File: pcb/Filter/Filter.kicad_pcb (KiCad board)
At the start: 2 copper layers, 100 x 100 mm, 8 parts, among them J1 Conn_01x01, J2 Conn_01x01, J3 Conn_01x02

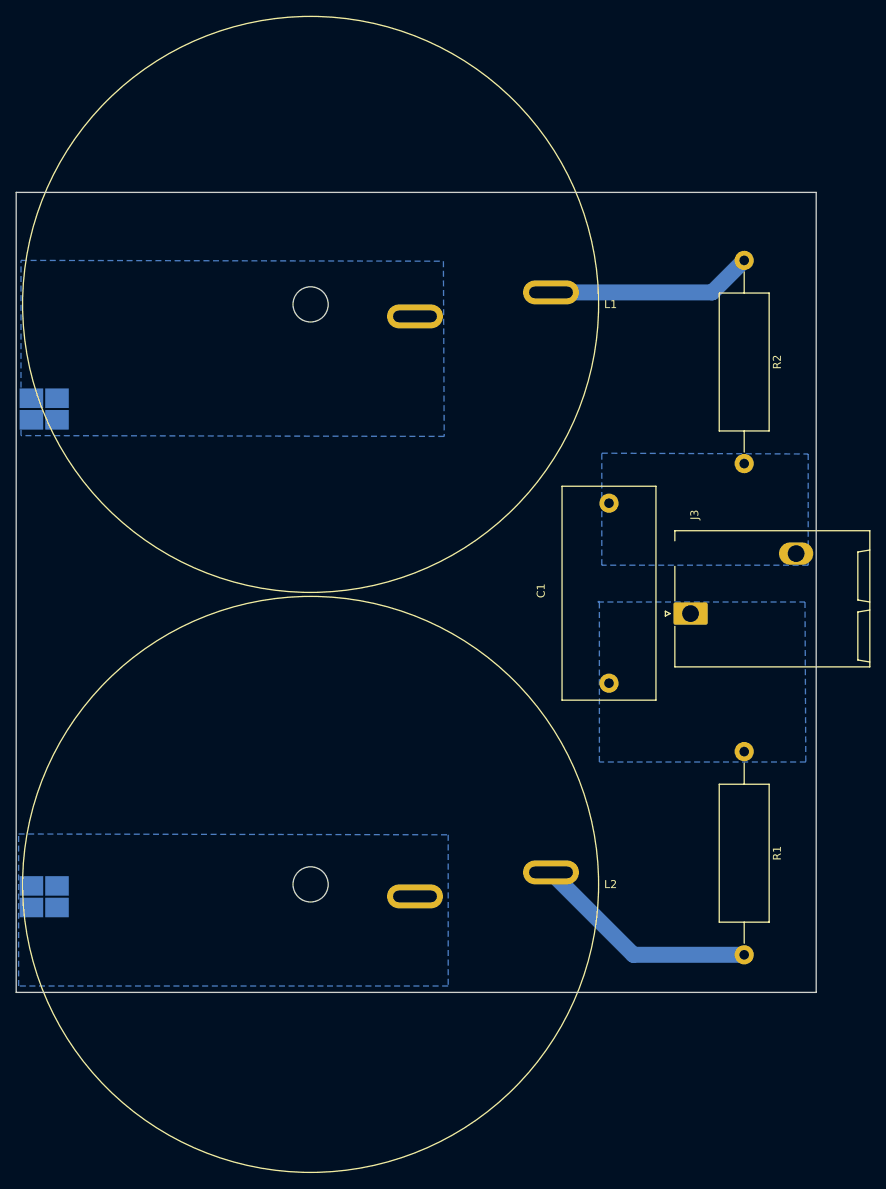
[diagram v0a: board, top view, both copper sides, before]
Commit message: filter + backplane
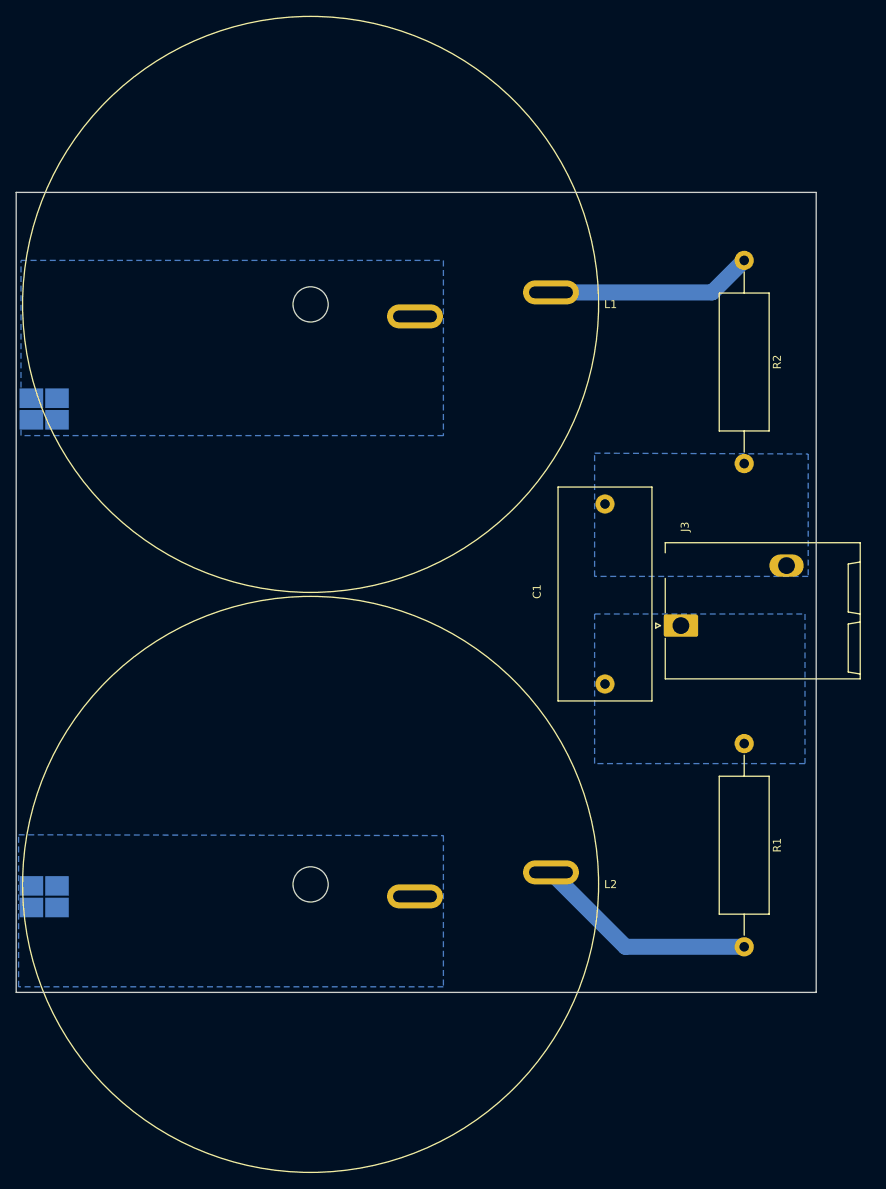
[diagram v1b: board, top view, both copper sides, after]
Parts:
- moved J3 1.92 mm to (123.1, 114.2)
- moved R1 1.00 mm to (131.0, 128.9)
- moved C1 0.51 mm to (113.6, 99.0)
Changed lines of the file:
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@@
 	(footprint "Resistor_THT:R_Axial_DIN0617_L17.0mm_D6.0mm_P25.40mm_Horizontal"
 		(layer "F.Cu")
-		(at 131 129.9 -90)
+		(at 131 128.9 -90)
 		(descr "Resistor, Axial_DIN0617 series, Axial, Horizontal, pin pitch=25.4mm, 2W, length*diameter=17*6mm^2, http://www.vishay.com/docs/20128/wkxwrx.pdf")
 		(tags "Resistor Axial_DIN0617 series Axial Horizontal pin pitch 25.4mm 2W length 17mm diameter 6mm")
@@
 	(footprint "Capacitor_THT:C_Rect_L26.5mm_W11.5mm_P22.50mm_MKS4"
 		(layer "F.Cu")
-		(at 114.1 98.85 -90)
+		(at 113.6 98.95 -90)
 		(descr "C, Rect series, Radial, pin pitch=22.50mm, , length*width=26.5*11.5mm^2, Capacitor, http://www.wima.com/EN/WIMA_MKS_4.pdf")
 		(tags "C Rect series Radial pin pitch 22.50mm  length 26.5mm width 11.5mm Capacitor")
@@
 	(footprint "Connector_Phoenix_SPT:PhoenixContact_SPT_5_2-H-7.5-ZB_1x02_P7.5mm_Horizontal"
 		(layer "F.Cu")
-		(at 124.2925 112.65 90)
+		(at 123.0925 114.15 90)
 		(descr "Connector Phoenix Contact, SPT 5/2-H-7.5-ZB Terminal Block, 1719192 (https://www.phoenixcontact.com/online/portal/gb/?uri=pxc-oc-itemdetail:pid=1719192), generated with kicad-footprint-generator")
 		(tags "Connector Phoenix Contact SPT 5/2-H-7.5-ZB 1719192")
@@
 	)
 	(segment
-		(start 131 155.3)
-		(end 117.15 155.3)
+		(start 116.15 154.3)
+		(end 106.85 145)
 		(width 2)
 		(layer "B.Cu")
@@
 	)
 	(segment
-		(start 117.15 155.3)
-		(end 106.85 145)
+		(start 131 154.3)
+		(end 116.15 154.3)
 		(width 2)
 		(layer "B.Cu")
@@
 	)
 	(zone
+		(net 0)
+		(net_name "")
+		(layers "F&B.Cu" "Edge.Cuts")
+		(hatch edge 0.5)
+		(connect_pads
+			(clearance 0)
+		)
+		(min_thickness 0.25)
+		(filled_areas_thickness no)
+		(keepout
+			(tracks not_allowed)
+			(vias allowed)
+			(pads allowed)
+			(copperpour not_allowed)
+			(footprints allowed)
+		)
+		(fill
+			(thermal_gap 0.5)
+			(thermal_bridge_width 0.5)
+		)
+		(polygon
+			(pts
+				(xy 73.1 142.8) (xy 80.4 142.8) (xy 80.4 150) (xy 73.1 150)
+			)
+		)
+	)
+	(zone
+		(net 0)
+		(net_name "")
+		(layers "F&B.Cu" "Edge.Cuts")
+		(hatch edge 0.5)
+		(connect_pads
+			(clearance 0)
+		)
+		(min_thickness 0.25)
+		(filled_areas_thickness no)
+		(keepout
+			(tracks not_allowed)
+			(vias allowed)
+			(pads allowed)
+			(copperpour not_allowed)
+			(footprints allowed)
+		)
+		(fill
+			(thermal_gap 0.5)
+			(thermal_bridge_width 0.5)
+		)
+		(polygon
+			(pts
+				(xy 73.2 70.4) (xy 80.5 70.4) (xy 80.5 77.6) (xy 73.2 77.6)
+			)
+		)
+	)
+	(zone
 		(net 2)
 		(net_name "/phb")
@@
 		(polygon
 			(pts
-				(xy 40.3 140.2) (xy 94 140.3) (xy 94 159.2) (xy 40.3 159.2)
+				(xy 40.3 140.3) (xy 93.4 140.4) (xy 93.4 159.3) (xy 40.3 159.3)
 			)
 		)
@@
 		(polygon
 			(pts
-				(xy 112.7 111.2) (xy 138.6 111.2) (xy 138.7 131.2) (xy 112.9 131.2) (xy 112.9 111.1)
+				(xy 112.3 112.7) (xy 138.6 112.7) (xy 138.6 131.4) (xy 112.3 131.4)
 			)
 		)
@@
 		(polygon
 			(pts
-				(xy 40.6 68.5) (xy 93.4 68.6) (xy 93.5 90.5) (xy 40.6 90.4)
+				(xy 40.6 68.5) (xy 93.4 68.5) (xy 93.4 90.4) (xy 40.6 90.4)
 			)
 		)
@@
 		(polygon
 			(pts
-				(xy 113.2 92.6) (xy 139 92.7) (xy 139 106.6) (xy 113.2 106.6) (xy 113.2 92.6)
-			)
-		)
+				(xy 112.3 92.6) (xy 139 92.7) (xy 139 108) (xy 112.3 108)
+			)
+		)
